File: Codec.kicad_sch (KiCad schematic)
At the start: 14 parts

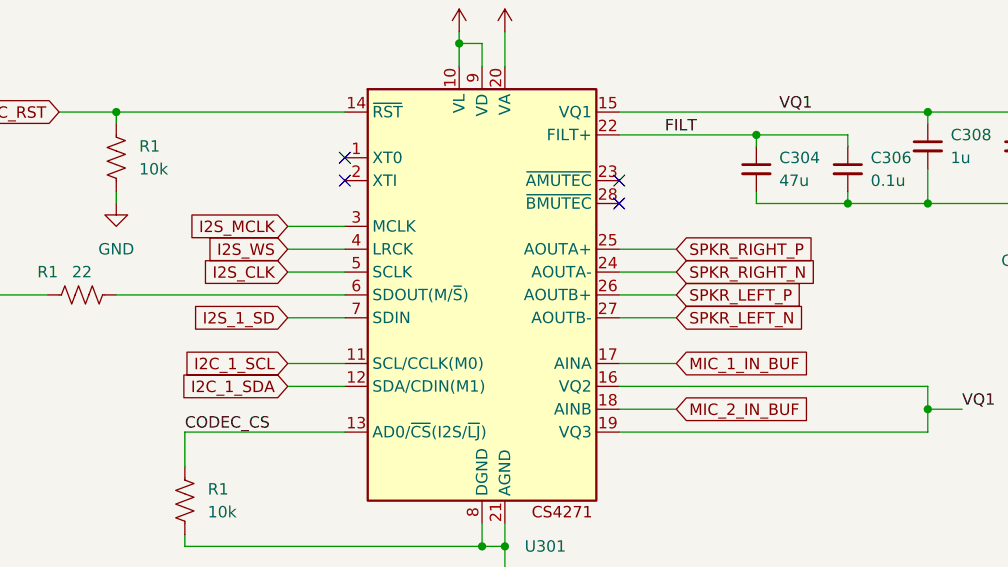
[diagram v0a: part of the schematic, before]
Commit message: ara ara
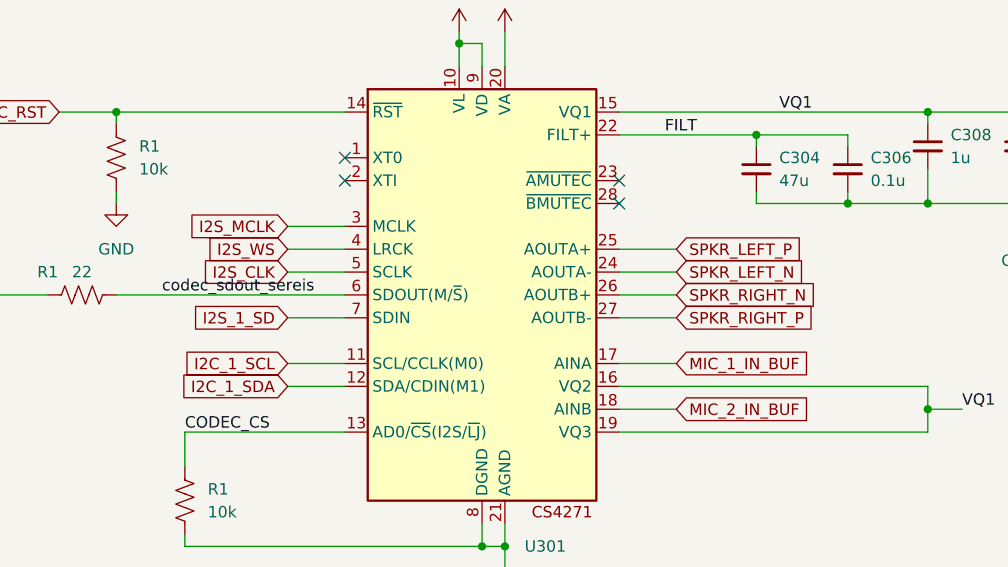
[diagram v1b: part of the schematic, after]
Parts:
- R1: footprint Resistor_SMD:R_0612_1632Metric_Pad1.18x3.40mm_HandSolder -> Resistor_SMD:R_0402_1005Metric_Pad0.72x0.64mm_HandSolder
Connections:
- net SPKR_LEFT_N: now also U301.24 (AOUTA-); no longer U301.27 (AOUTB-)
- net SPKR_LEFT_P: now also U301.25 (AOUTA+); no longer U301.26 (AOUTB+)
- net SPKR_RIGHT_N: now also U301.26 (AOUTB+); no longer U301.24 (AOUTA-)
- net SPKR_RIGHT_P: now also U301.27 (AOUTB-); no longer U301.25 (AOUTA+)
- net codec_sdout_sereis: now reaches R1.2, U301.6 (SDOUT(M/~{S}))
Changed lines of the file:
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@@
     (stroke (width 0) (type default))
   )
+  (label "codec_sdout_sereis" (at 162.56 100.33 0) (fields_autoplaced)
+    (effects (font (size 1.27 1.27)) (justify left bottom))
+  )
   (label "VQ1" (at 231.14 80.01 0) (fields_autoplaced)
     (effects (font (size 1.27 1.27)) (justify left bottom))
@@
     (effects (font (size 1.27 1.27)) (justify left bottom))
   )
-  (global_label "SPKR_LEFT_N" (shape input) (at 219.71 102.87 0) (fields_autoplaced)
-    (effects (font (size 1.27 1.27)) (justify left))
-    (property "Intersheetrefs" "${INTERSHEET_REFS}" (at 235.2137 102.87 0)
-      (effects (font (size 1.27 1.27)) (justify left) hide)
-    )
-  )
-  (global_label "SPKR_RIGHT_P" (shape input) (at 219.71 95.25 0) (fields_autoplaced)
-    (effects (font (size 1.27 1.27)) (justify left))
-    (property "Intersheetrefs" "${INTERSHEET_REFS}" (at 236.3628 95.25 0)
-      (effects (font (size 1.27 1.27)) (justify left) hide)
-    )
-  )
   (global_label "MIC_1_IN_BUF" (shape input) (at 219.71 107.95 0) (fields_autoplaced)
     (effects (font (size 1.27 1.27)) (justify left))
@@
     )
   )
+  (global_label "SPKR_LEFT_N" (shape input) (at 219.71 97.79 0) (fields_autoplaced)
+    (effects (font (size 1.27 1.27)) (justify left))
+    (property "Intersheetrefs" "${INTERSHEET_REFS}" (at 235.2137 97.79 0)
+      (effects (font (size 1.27 1.27)) (justify left) hide)
+    )
+  )
+  (global_label "SPKR_LEFT_P" (shape input) (at 219.71 95.25 0) (fields_autoplaced)
+    (effects (font (size 1.27 1.27)) (justify left))
+    (property "Intersheetrefs" "${INTERSHEET_REFS}" (at 235.1532 95.25 0)
+      (effects (font (size 1.27 1.27)) (justify left) hide)
+    )
+  )
   (global_label "MIC_2_IN_BUF" (shape input) (at 219.71 113.03 0) (fields_autoplaced)
     (effects (font (size 1.27 1.27)) (justify left))
@@
     )
   )
+  (global_label "SPKR_RIGHT_P" (shape input) (at 219.71 102.87 0) (fields_autoplaced)
+    (effects (font (size 1.27 1.27)) (justify left))
+    (property "Intersheetrefs" "${INTERSHEET_REFS}" (at 236.3628 102.87 0)
+      (effects (font (size 1.27 1.27)) (justify left) hide)
+    )
+  )
   (global_label "I2S_MCLK" (shape input) (at 176.53 92.71 180) (fields_autoplaced)
     (effects (font (size 1.27 1.27)) (justify right))
@@
     )
   )
-  (global_label "SPKR_RIGHT_N" (shape input) (at 219.71 97.79 0) (fields_autoplaced)
-    (effects (font (size 1.27 1.27)) (justify left))
-    (property "Intersheetrefs" "${INTERSHEET_REFS}" (at 236.4233 97.79 0)
+  (global_label "SPKR_RIGHT_N" (shape input) (at 219.71 100.33 0) (fields_autoplaced)
+    (effects (font (size 1.27 1.27)) (justify left))
+    (property "Intersheetrefs" "${INTERSHEET_REFS}" (at 236.4233 100.33 0)
       (effects (font (size 1.27 1.27)) (justify left) hide)
     )
@@
     (property "Intersheetrefs" "${INTERSHEET_REFS}" (at 137.4406 80.01 0)
       (effects (font (size 1.27 1.27)) (justify right) hide)
-    )
-  )
-  (global_label "SPKR_LEFT_P" (shape input) (at 219.71 100.33 0) (fields_autoplaced)
-    (effects (font (size 1.27 1.27)) (justify left))
-    (property "Intersheetrefs" "${INTERSHEET_REFS}" (at 235.1532 100.33 0)
-      (effects (font (size 1.27 1.27)) (justify left) hide)
     )
   )
@@
       (effects (font (size 1.27 1.27)) (justify left))
     )
-    (property "Footprint" "Resistor_SMD:R_0612_1632Metric_Pad1.18x3.40mm_HandSolder" (at 166.116 123.444 90)
+    (property "Footprint" "Resistor_SMD:R_0402_1005Metric_Pad0.72x0.64mm_HandSolder" (at 166.116 123.444 90)
       (effects (font (size 1.27 1.27)) hide)
     )
@@
       (effects (font (size 1.27 1.27)) (justify left))
     )
-    (property "Footprint" "Resistor_SMD:R_0612_1632Metric_Pad1.18x3.40mm_HandSolder" (at 158.496 85.344 90)
-      (effects (font (size 1.27 1.27)) hide)
-    )
+    (property "Footprint" "Resistor_SMD:R_0402_1005Metric_Pad0.72x0.64mm_HandSolder" (at 158.496 85.344 90)
+      (effects (font (size 1.27 1.27)) hide)
+    )
